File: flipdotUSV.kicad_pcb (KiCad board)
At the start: 2 copper layers, 65 x 56.5 mm, 34 parts, among them IC1 ATTINY13-S, P2 CONN_01X02, P3 Raspberry_Pi_+_Conn, P4 CONN_01X02, Q1 BC547, U1 LM2596S-5

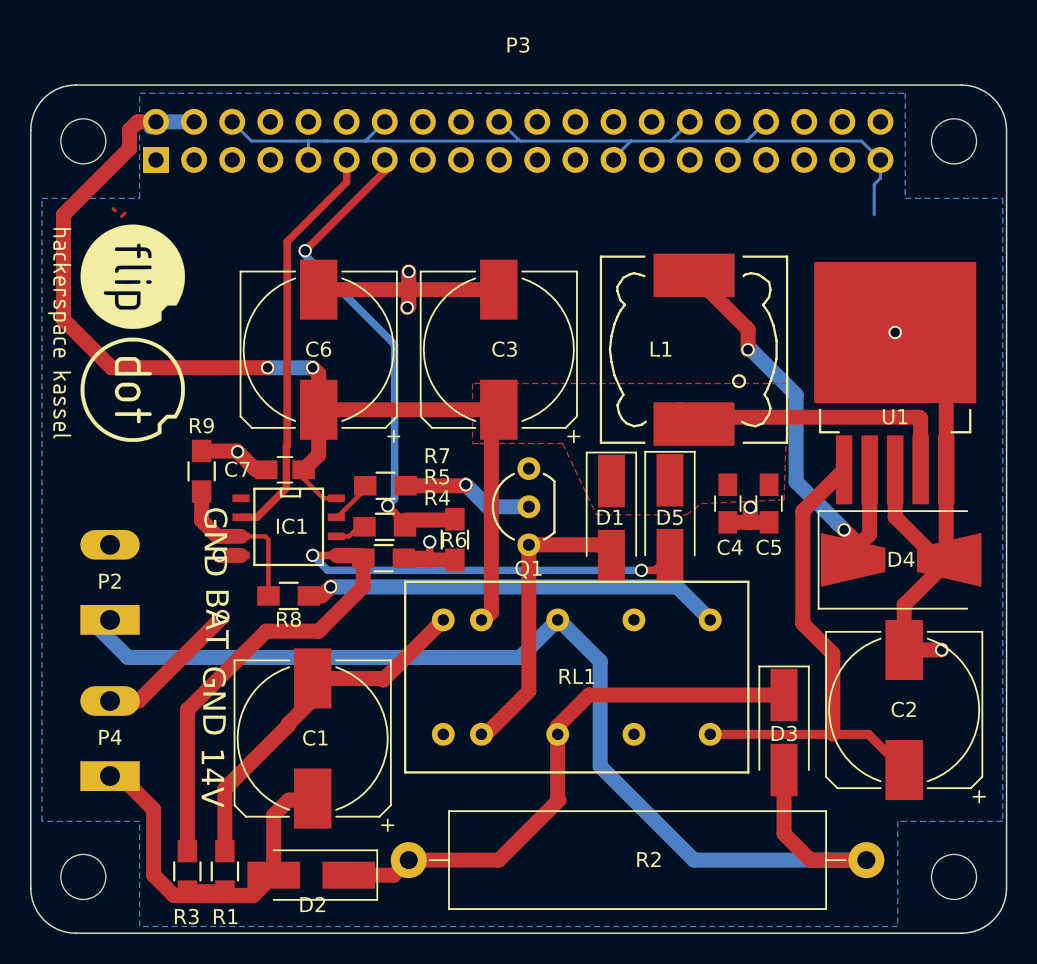
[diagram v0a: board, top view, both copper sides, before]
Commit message: fixed footprint fuckup
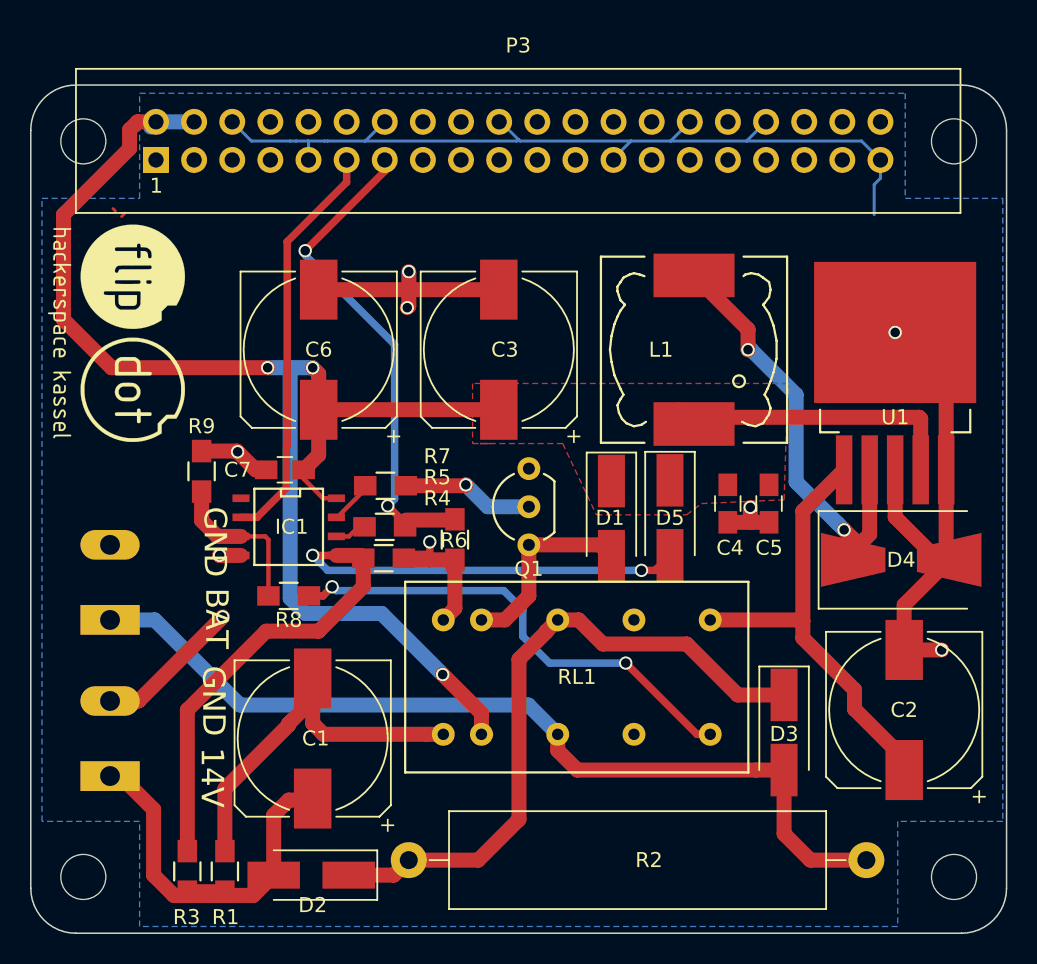
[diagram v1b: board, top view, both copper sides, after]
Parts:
- P2, P4: footprint smd_proto:AK300-2_without -> Connect:AK300-2; moved to B.Cu
- P3: footprint smd_proto:IDC_Header_Straight_40pins_without -> Connect:IDC_Header_Straight_40pins
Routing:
- net +5V: track 94.7 -> 113.8 mm, vias 2 -> 3
- net +BATT: track 74.9 -> 60.1 mm
- net Net-(D2-Pad1): track 37.0 -> 44.5 mm
- net Rel_off: track 19.9 -> 13.2 mm
- net GND: track 132.8 -> 137.1 mm
- net Batt_Voltage: track 27.9 -> 32.1 mm, vias 1 -> 2
- net Net-(C2-Pad1): track 33.5 -> 30.1 mm
- net Net-(C1-Pad2): track 24.3 -> 25.9 mm
